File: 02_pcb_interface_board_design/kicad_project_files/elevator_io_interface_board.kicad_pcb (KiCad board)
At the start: 2 copper layers, 94.2 x 102 mm, 60 parts, among them J1 Power Input, J10 MCU Output Header, J11 Motor UP Output, J12 Motor DOWN Output, J13 Door OPEN Output, J14 Door CLOSE Output, J15 SWD_IO, J2 MCU Input Header, J3 Floor 1 Button, J4 Floor 2 Button, J5 Floor 3 Button, J6 Door Sensor, J7 Emergency Stop, J8 Upper Limit Switch, J9 Lower Limit Switch, K1 Relay_SPDT, K2 Relay_SPDT, K3 Relay_SPDT, K4 Relay_SPDT, Q1 2N2222, Q2 2N2222, Q3 2N2222, Q4 2N2222, SW1 SW_Push, SW2 SW_SPDT, U1 STM32F103C8T6, U2 AMS1117-3.3

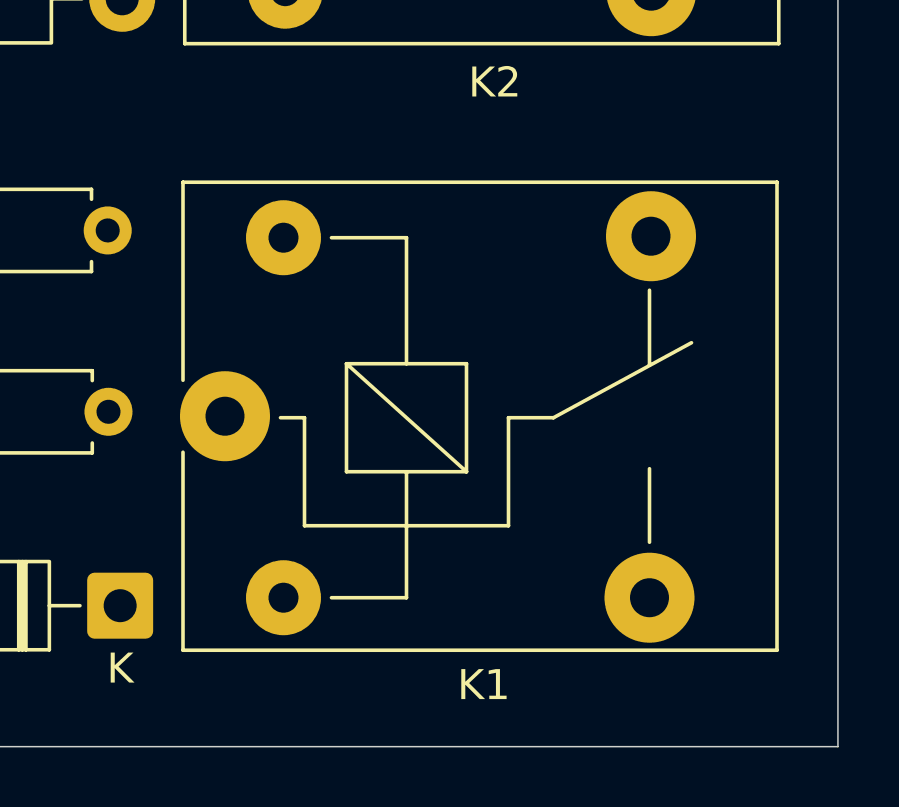
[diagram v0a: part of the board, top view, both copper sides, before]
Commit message: PCB Design finalized!
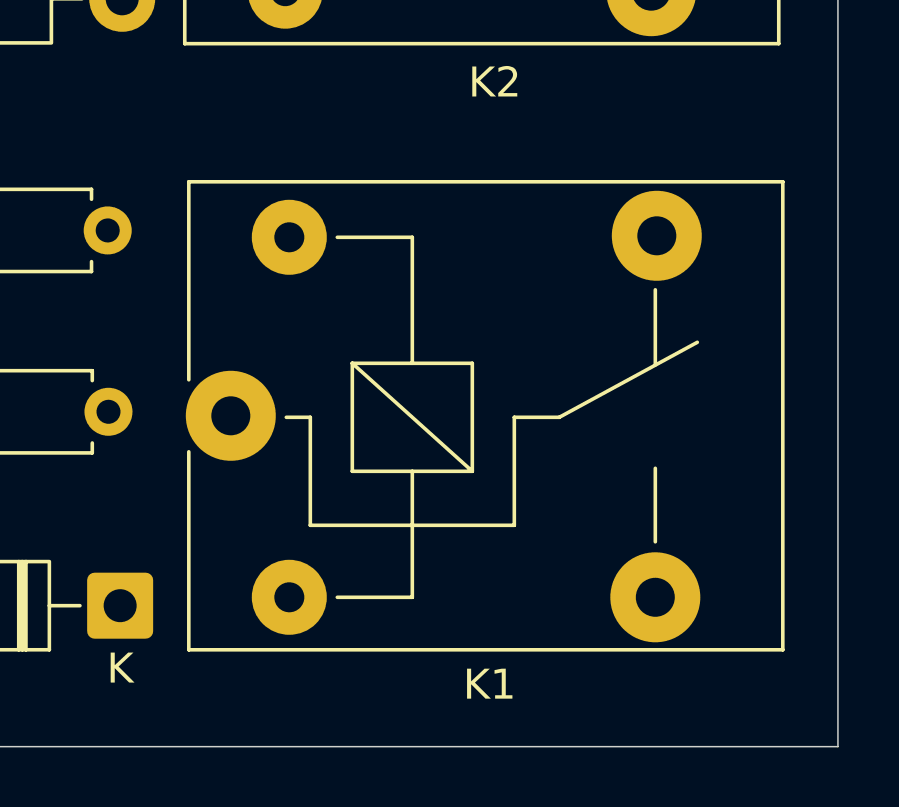
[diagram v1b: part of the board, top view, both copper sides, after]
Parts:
- moved K1 0.19 mm to (144.8, 164.5)
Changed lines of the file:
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@@
 	(footprint "Relay_THT:Relay_SPDT_SANYOU_SRD_Series_Form_C"
 		(layer "F.Cu")
-		(at 144.592 164.5506)
+		(at 144.7858 164.5364)
 		(descr "relay Sanyou SRD series Form C http://www.sanyourelay.ca/public/products/pdf/SRD.pdf")
 		(tags "relay Sanyu SRD form C")
